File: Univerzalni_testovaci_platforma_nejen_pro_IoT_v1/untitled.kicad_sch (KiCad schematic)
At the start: 6 parts, among them J1 Conn_01x22_Female ESP S3 J1, J2 Conn_01x22_Female ESP S3 J3, J3 Conn_01x19_Female ESP DEV_KIT, J4 Conn_01x19_Female ESP DEV_KIT, U1 ESP32-S3

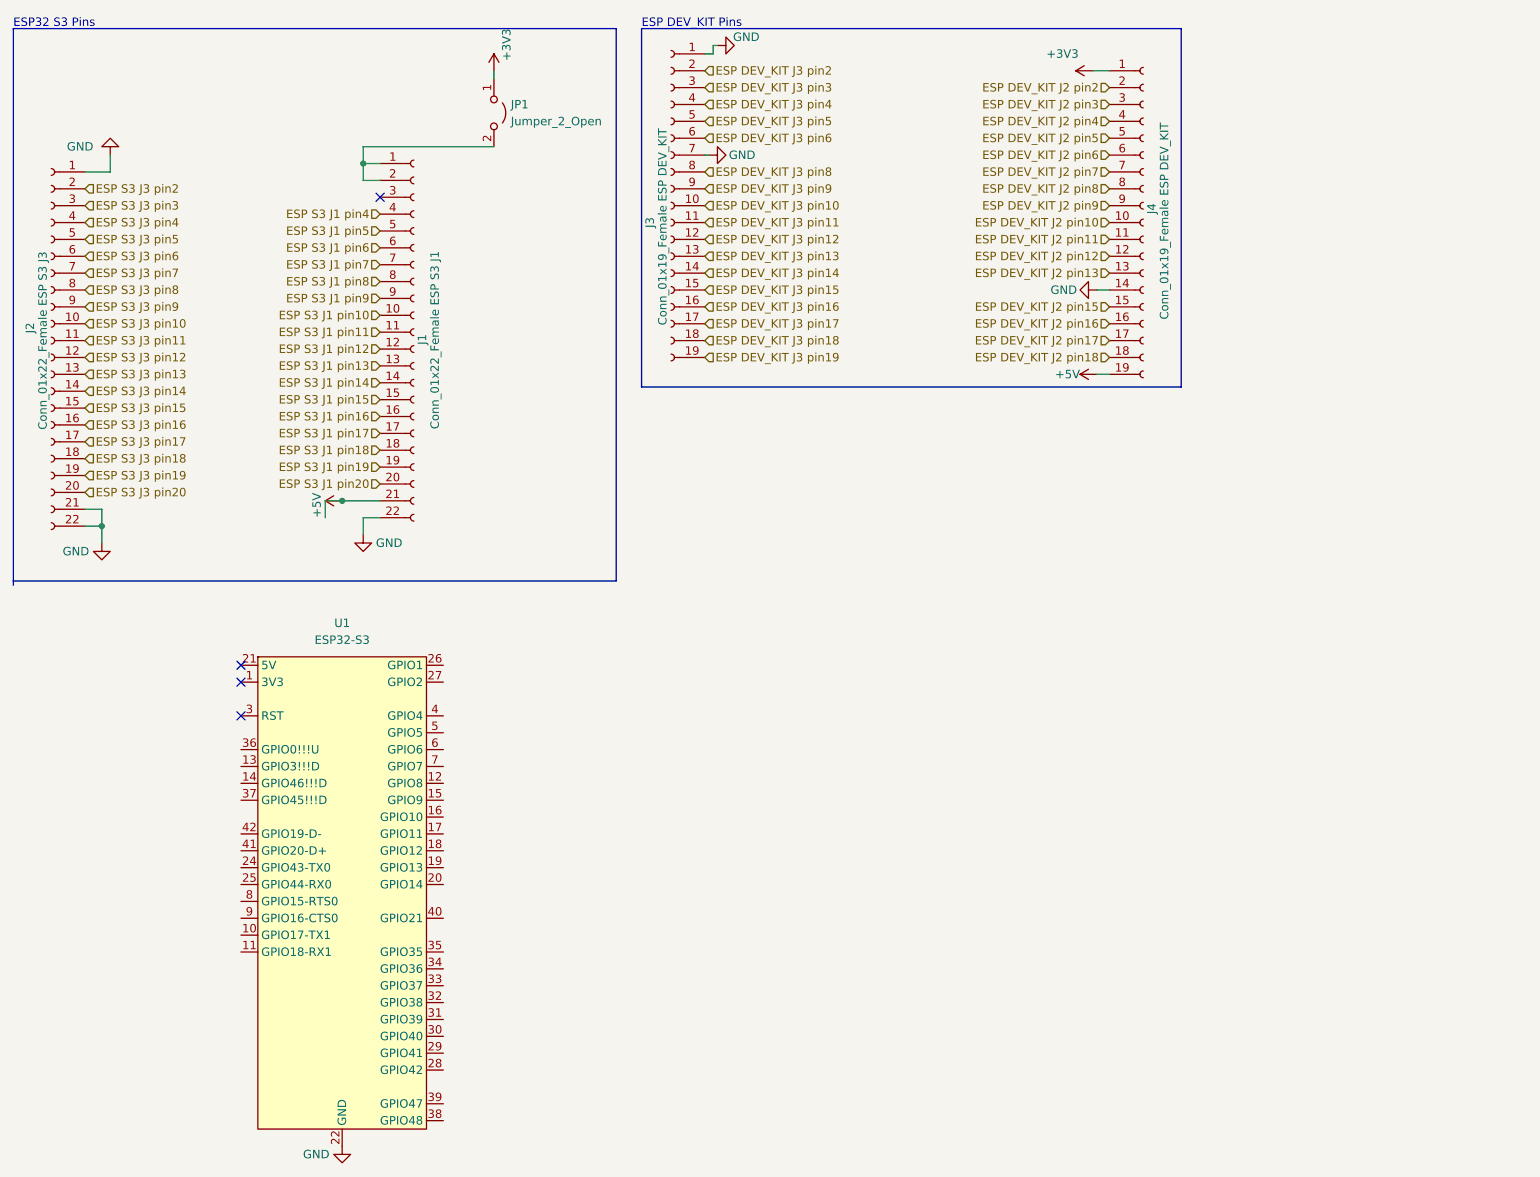
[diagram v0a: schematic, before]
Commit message: schema hotovo
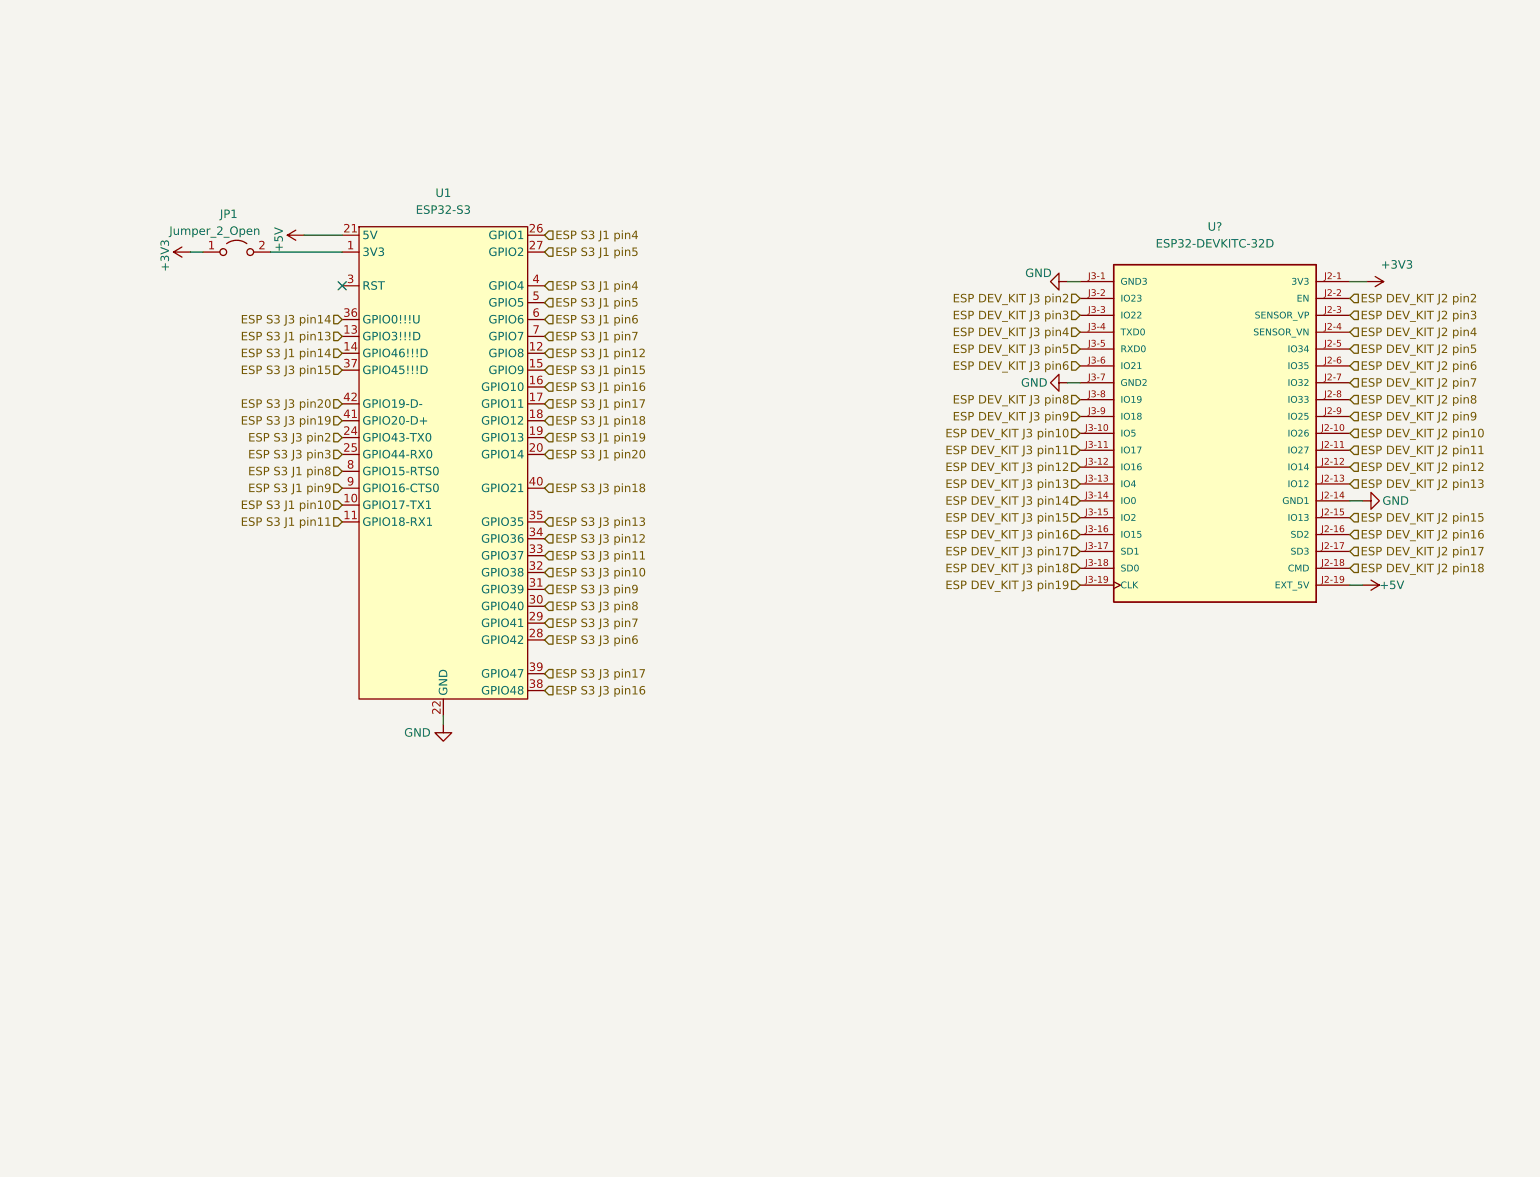
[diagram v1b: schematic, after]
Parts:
- removed J1: Conn_01x22_Female ESP S3 J1, Connector_PinSocket_2.54mm:PinSocket_1x22_P2.54mm_Vertical, symbol Connector:Conn_01x22_Female
- removed J2: Conn_01x22_Female ESP S3 J3, Connector_PinSocket_2.54mm:PinSocket_1x22_P2.54mm_Vertical, symbol Connector:Conn_01x22_Female
- removed J3, J4: Conn_01x19_Female ESP DEV_KIT, Connector_PinSocket_2.54mm:PinSocket_1x19_P2.54mm_Vertical, symbol Connector:Conn_01x19_Female
- added U?: ESP32-DEVKITC-32D, ESP32-DEVKITC-32D:MODULE_ESP32-DEVKITC-32D, symbol robotarna_sym:ESP32-DEVKITC-32D
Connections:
- net +3V3: now also U?.J2-1 (3V3)
- net +5V: now also U1.21 (5V), U?.J2-19 (EXT_5V)
- net ESP DEV_KIT J2 pin10: now also U?.J2-10 (IO26)
- net ESP DEV_KIT J2 pin11: now also U?.J2-11 (IO27)
- net ESP DEV_KIT J2 pin12: now also U?.J2-12 (IO14)
- net ESP DEV_KIT J2 pin13: now also U?.J2-13 (IO12)
- net ESP DEV_KIT J2 pin15: now also U?.J2-15 (IO13)
- net ESP DEV_KIT J2 pin16: now also U?.J2-16 (SD2)
- net ESP DEV_KIT J2 pin17: now also U?.J2-17 (SD3)
- net ESP DEV_KIT J2 pin18: now also U?.J2-18 (CMD)
- net ESP DEV_KIT J2 pin2: now also U?.J2-2 (EN)
- net ESP DEV_KIT J2 pin3: now also U?.J2-3 (SENSOR_VP)
- net ESP DEV_KIT J2 pin4: now also U?.J2-4 (SENSOR_VN)
- net ESP DEV_KIT J2 pin5: now also U?.J2-5 (IO34)
- net ESP DEV_KIT J2 pin6: now also U?.J2-6 (IO35)
- net ESP DEV_KIT J2 pin7: now also U?.J2-7 (IO32)
- net ESP DEV_KIT J2 pin8: now also U?.J2-8 (IO33)
- net ESP DEV_KIT J2 pin9: now also U?.J2-9 (IO25)
- net ESP DEV_KIT J3 pin10: now also U?.J3-10 (IO5)
- net ESP DEV_KIT J3 pin11: now also U?.J3-11 (IO17)
- net ESP DEV_KIT J3 pin12: now also U?.J3-12 (IO16)
- net ESP DEV_KIT J3 pin13: now also U?.J3-13 (IO4)
- net ESP DEV_KIT J3 pin14: now also U?.J3-14 (IO0)
- net ESP DEV_KIT J3 pin15: now also U?.J3-15 (IO2)
- net ESP DEV_KIT J3 pin16: now also U?.J3-16 (IO15)
- net ESP DEV_KIT J3 pin17: now also U?.J3-17 (SD1)
- net ESP DEV_KIT J3 pin18: now also U?.J3-18 (SD0)
- net ESP DEV_KIT J3 pin19: now also U?.J3-19 (CLK)
- net ESP DEV_KIT J3 pin2: now also U?.J3-2 (IO23)
- net ESP DEV_KIT J3 pin3: now also U?.J3-3 (IO22)
- net ESP DEV_KIT J3 pin4: now also U?.J3-4 (TXD0)
- net ESP DEV_KIT J3 pin5: now also U?.J3-5 (RXD0)
- net ESP DEV_KIT J3 pin6: now also U?.J3-6 (IO21)
- net ESP DEV_KIT J3 pin8: now also U?.J3-8 (IO19)
- net ESP DEV_KIT J3 pin9: now also U?.J3-9 (IO18)
- net ESP S3 J1 pin10: now also U1.10 (GPIO17-TX1)
- net ESP S3 J1 pin11: now also U1.11 (GPIO18-RX1)
- net ESP S3 J1 pin12: now also U1.12 (GPIO8)
- net ESP S3 J1 pin13: now also U1.13 (GPIO3!!!D)
- net ESP S3 J1 pin14: now also U1.14 (GPIO46!!!D)
- net ESP S3 J1 pin15: now also U1.15 (GPIO9)
- net ESP S3 J1 pin16: now also U1.16 (GPIO10)
- net ESP S3 J1 pin17: now also U1.17 (GPIO11)
- net ESP S3 J1 pin18: now also U1.18 (GPIO12)
- net ESP S3 J1 pin19: now also U1.19 (GPIO13)
- net ESP S3 J1 pin20: now also U1.20 (GPIO14)
- net ESP S3 J1 pin4: now also U1.26 (GPIO1), U1.4 (GPIO4)
- net ESP S3 J1 pin5: now also U1.27 (GPIO2), U1.5 (GPIO5)
- net ESP S3 J1 pin6: now also U1.6 (GPIO6)
- net ESP S3 J1 pin7: now also U1.7 (GPIO7)
- net ESP S3 J1 pin8: now also U1.8 (GPIO15-RTS0)
- net ESP S3 J1 pin9: now also U1.9 (GPIO16-CTS0)
- net ESP S3 J3 pin10: now also U1.32 (GPIO38)
- net ESP S3 J3 pin11: now also U1.33 (GPIO37)
- net ESP S3 J3 pin12: now also U1.34 (GPIO36)
- net ESP S3 J3 pin13: now also U1.35 (GPIO35)
- net ESP S3 J3 pin14: now also U1.36 (GPIO0!!!U)
- net ESP S3 J3 pin15: now also U1.37 (GPIO45!!!D)
- net ESP S3 J3 pin16: now also U1.38 (GPIO48)
- net ESP S3 J3 pin17: now also U1.39 (GPIO47)
- net ESP S3 J3 pin18: now also U1.40 (GPIO21)
- net ESP S3 J3 pin19: now also U1.41 (GPIO20-D+)
- net ESP S3 J3 pin2: now also U1.24 (GPIO43-TX0)
- net ESP S3 J3 pin20: now also U1.42 (GPIO19-D-)
- net ESP S3 J3 pin3: now also U1.25 (GPIO44-RX0)
- net ESP S3 J3 pin6: now also U1.28 (GPIO42)
- net ESP S3 J3 pin7: now also U1.29 (GPIO41)
- net ESP S3 J3 pin8: now also U1.30 (GPIO40)
- net ESP S3 J3 pin9: now also U1.31 (GPIO39)
- net GND: now also U?.J2-14 (GND1), U?.J3-1 (GND3), U?.J3-7 (GND2)
- net at U1.1 (3V3), U1.2 (3V3): now also JP1.2 (B)
- no-connect marks 4 -> 1
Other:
- note removed: "ESP DEV_KIT Pins"
- note removed: "ESP32 S3 Pins"
- moved on the sheet: JP1, U1
